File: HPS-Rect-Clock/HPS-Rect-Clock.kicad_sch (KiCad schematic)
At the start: 38 parts, among them J1 Conn_01x06, J2 PJ-102AH, Y1 Crystal_16MHz

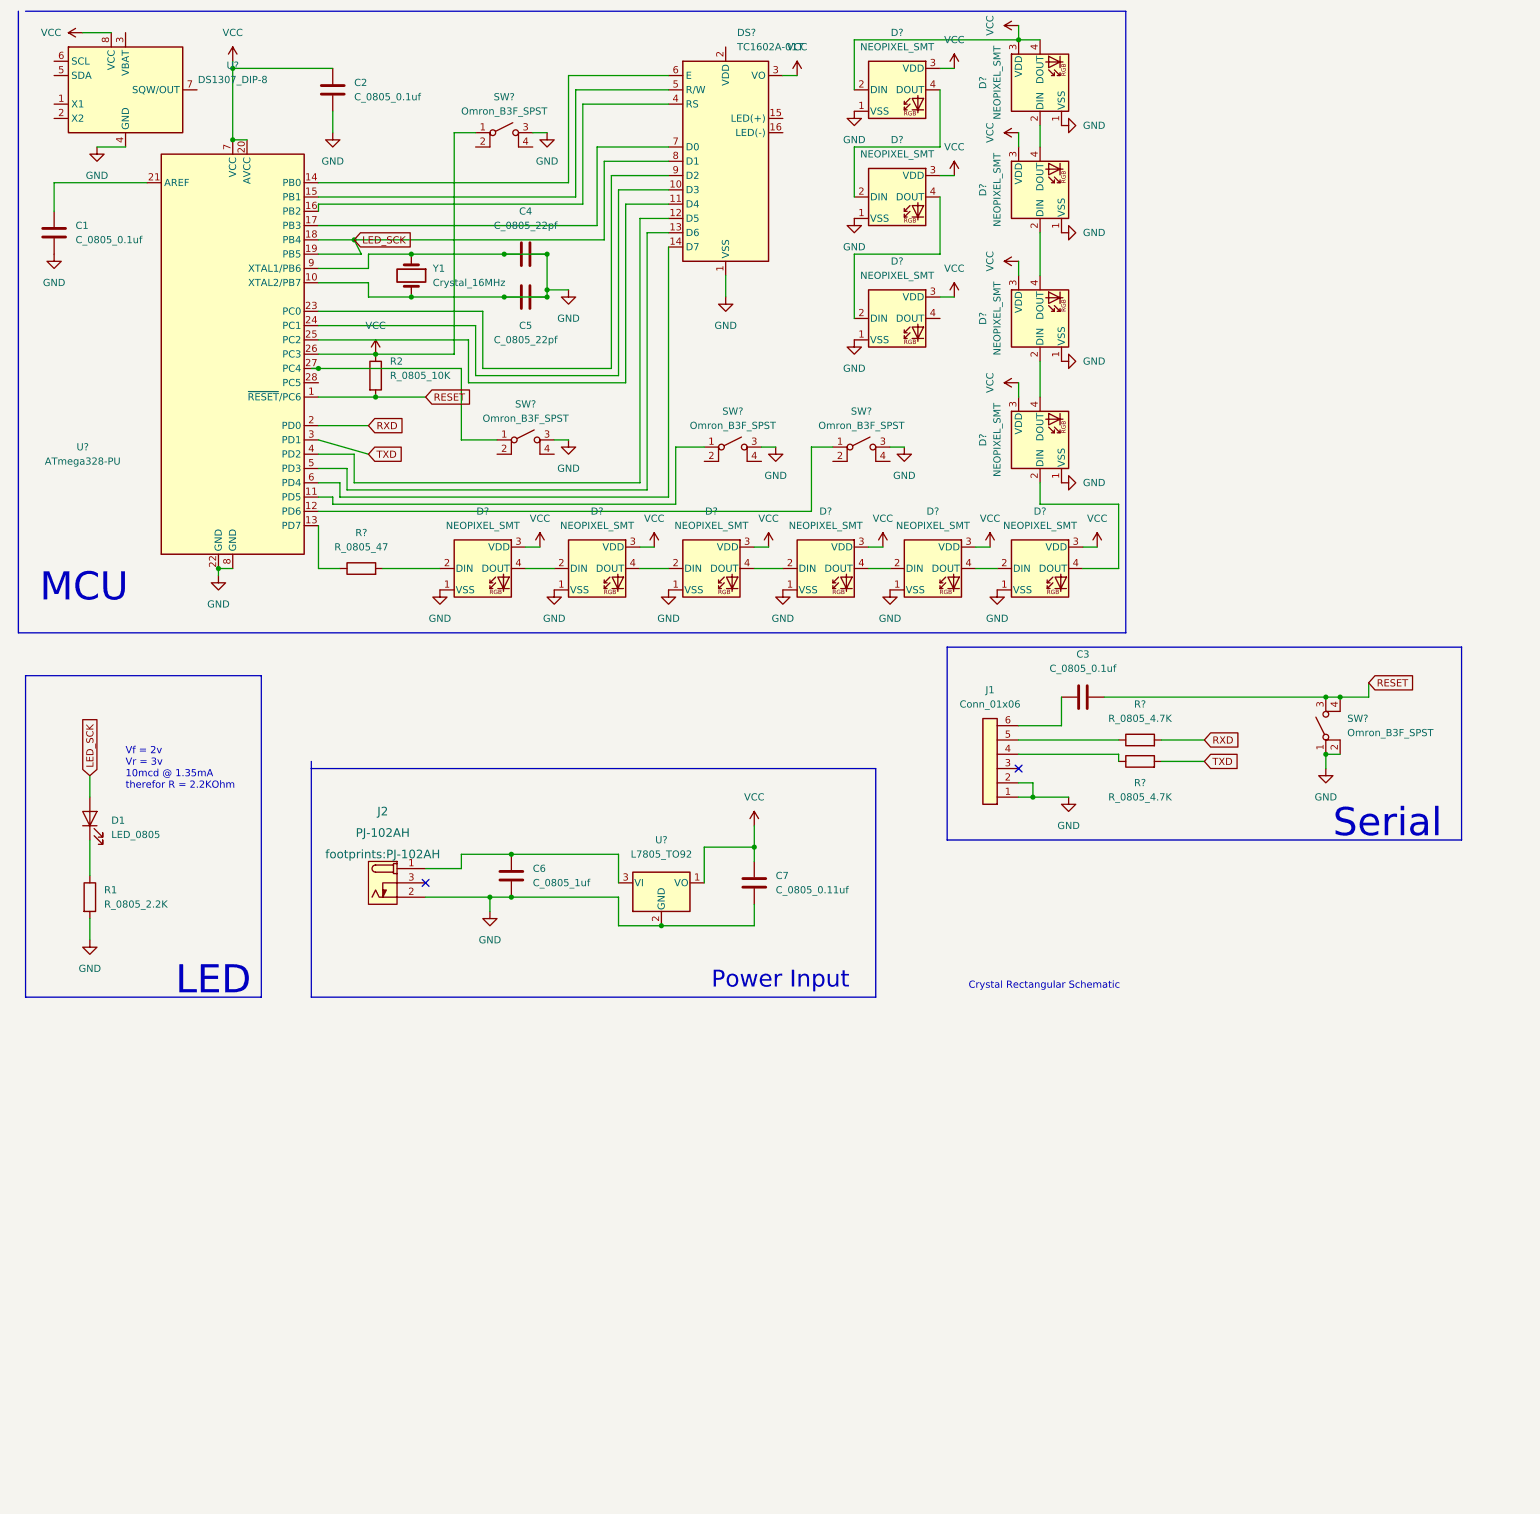
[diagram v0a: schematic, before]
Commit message: Week 5
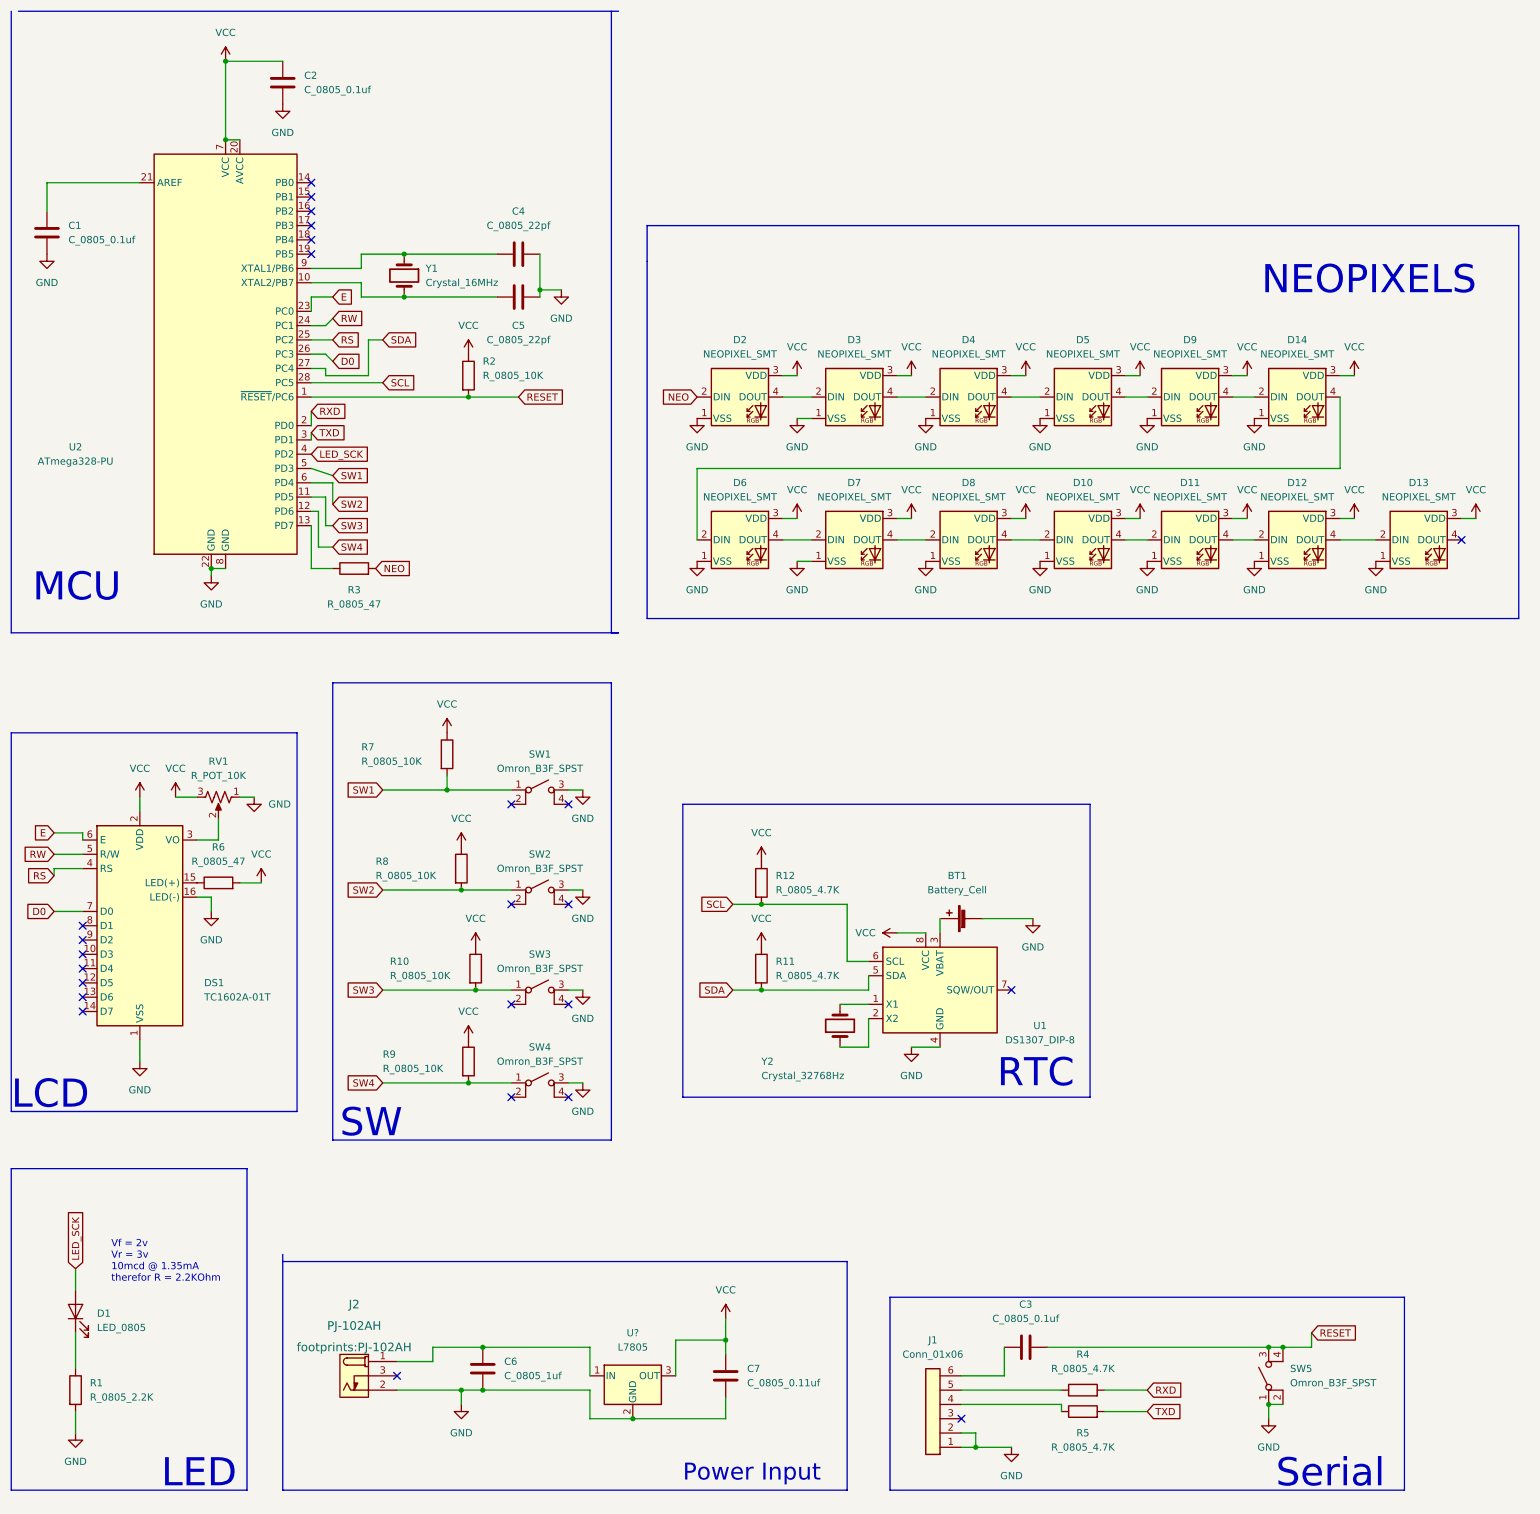
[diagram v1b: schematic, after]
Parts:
- removed D? (x7): NEOPIXEL_SMT, footprints:LED_SK6812_PLCC4_5.0x5.0mm_P3.2mm, symbol HPS:NEOPIXEL_SMT
- removed U?: L7805_TO92, footprints:TO-92_Inline, symbol HPS:L7805_TO92
- added BT1: Battery_Cell, footprints:BatteryHolder_Keystone_106_1x20mm, symbol HPS:Battery_Cell
- added D10, D11, D12, D13, D6, D7, D8: NEOPIXEL_SMT, footprints:LED_SK6812_PLCC4_5.0x5.0mm_P3.2mm, symbol HPS:NEOPIXEL_SMT
- added R10, R7, R8, R9: R_0805_10K, footprints:R_0805_2012Metric, symbol HPS:R_0805_10K
- added R11, R12: R_0805_4.7K, footprints:R_0805_2012Metric, symbol HPS:R_0805_4.7K
- added R6: R_0805_47, footprints:R_0805_2012Metric, symbol HPS:R_0805_47
- added RV1: R_POT_10K, footprints:Potentiometer_Bourns_3386P_Vertical, symbol HPS:R_POT_10K
- added U?: L7805, symbol HPS:L7805
- added Y2: Crystal_32768Hz, footprints:Crystal_SMD_2Pin_3.2x1.5mm, symbol HPS:Crystal_32768Hz
- gave numbers to parts that had none: 17
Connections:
- net GND: now also DS1.16 (LED(-)), BT1.2 (-), D10.1 (VSS), D11.1 (VSS), D12.1 (VSS), D13.1 (VSS), D6.1 (VSS), D7.1 (VSS), D8.1 (VSS), RV1.1, U?.2 (GND); no longer C4.1, C5.1, U2.10 (XTAL2/PB7), U2.9 (XTAL1/PB6), Y1.1, Y1.2
- net LED_SCK: now also U2.4 (PD2); no longer DS1.8 (D1), U2.18 (PB4), U2.19 (PB5)
- net VCC: now also DS1.2 (VDD), D10.3 (VDD), D11.3 (VDD), D12.3 (VDD), D13.3 (VDD), D6.3 (VDD), D7.3 (VDD), D8.3 (VDD), R10.1, R11.1, R12.1, R6.2, R7.1, R8.1, R9.1, RV1.3, U?.3 (OUT); no longer DS1.3 (VO), SW1.1 (A), U2.26 (PC3)
- net at C6.2, J2.1 (POLE): now also U?.1 (IN)
- net at DS1.10 (D3): no longer U2.24 (PC1)
- net at DS1.11 (D4): no longer U2.25 (PC2)
- net at DS1.12 (D5): no longer U2.4 (PD2)
- net at DS1.13 (D6): no longer U2.5 (PD3)
- net at DS1.14 (D7): no longer U2.6 (PD4)
- net at DS1.15 (LED(+)): now also R6.1
- net at U2.16 (PB2): no longer DS1.4 (RS)
- net at U2.15 (PB1): no longer DS1.5 (R/W)
- net at U2.14 (PB0): no longer DS1.6 (E)
- net at U2.17 (PB3): no longer DS1.7 (D0)
- net at DS1.9 (D2): no longer U2.23 (PC0)
- net SW3: now reaches SW3.1 (A), U2.11 (PD5)
- net SW3: now also R10.2
- net SDA: now reaches U2.27 (PC4)
- net SDA: now also U1.5 (SDA), R11.2; no longer SW2.1 (A)
- net SW4: now reaches SW4.1 (A), U2.12 (PD6)
- net SW4: now also R9.2
- net at D14.4 (DOUT): now also D6.2 (DIN)
- net NEO: now reaches D2.2 (DIN), R3.2
- net SCL: now reaches U2.28 (PC5)
- net SCL: now also U1.6 (SCL), R12.2
- net at U1.1 (X1): now also Y2.2
- net at U1.2 (X2): now also Y2.1
- net at U1.3 (VBAT): now also BT1.1 (+)
- new net: D12.4 (DOUT), D13.2 (DIN)
- new net: DS1.3 (VO), RV1.2
- new net: D11.4 (DOUT), D12.2 (DIN)
- new net: D6.4 (DOUT), D7.2 (DIN)
- new net: D7.4 (DOUT), D8.2 (DIN)
- new net: C4.1, U2.9 (XTAL1/PB6), Y1.1
- new net: C5.1, U2.10 (XTAL2/PB7), Y1.2
- new net: D10.4 (DOUT), D11.2 (DIN)
- new net: D10.2 (DIN), D8.4 (DOUT)
- new net D0: DS1.7 (D0), U2.26 (PC3)
- new net E: DS1.6 (E), U2.23 (PC0)
- new net RS: DS1.4 (RS), U2.25 (PC2)
- new net RW: DS1.5 (R/W), U2.24 (PC1)
- new net SW1: R7.2, SW1.1 (A), U2.5 (PD3)
- new net SW2: R8.2, SW2.1 (A), U2.6 (PD4)
- no-connect marks 2 -> 25
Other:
- note added: "LCD"
- note added: "NEOPIXELS"
- note added: "RTC"
- note added: "SW"
- note removed: "Crystal Rectangular Schematic"
- moved on the sheet: C1, C2, C3, C4, C5, C6, C7, D1, D14, D2, D3, D4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
